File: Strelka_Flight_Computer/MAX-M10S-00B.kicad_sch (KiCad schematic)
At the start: 15 parts, among them IC2 MAX-M10S-00B

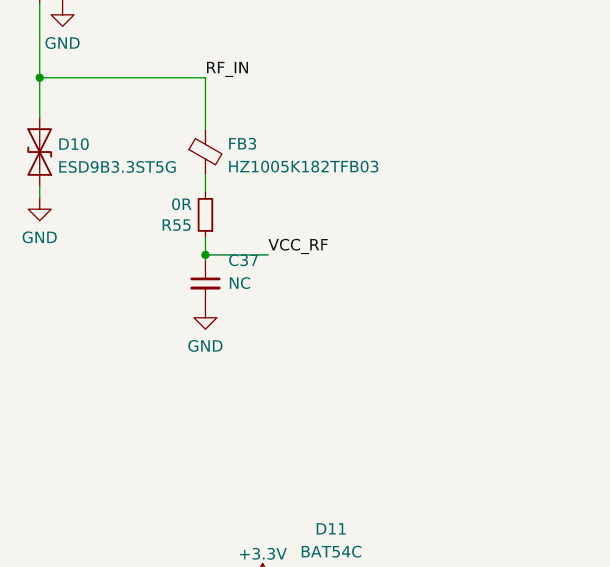
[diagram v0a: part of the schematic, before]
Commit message: Continued routing
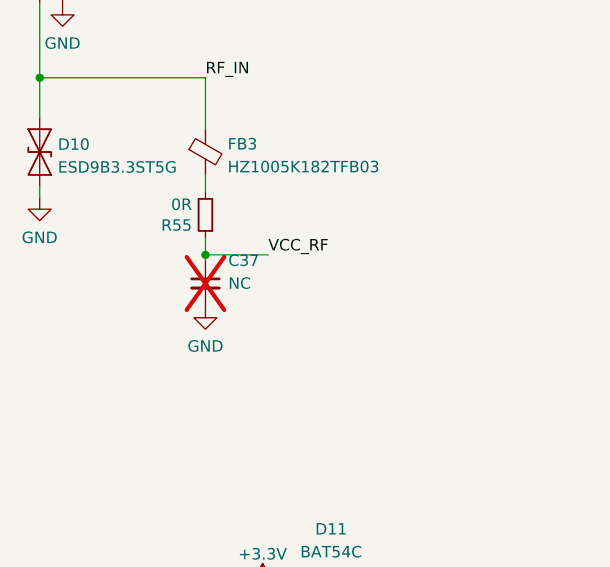
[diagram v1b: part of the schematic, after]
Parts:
- C37: now not fitted
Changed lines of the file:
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@@
   )
   (symbol (lib_id "Device:C_Small") (at 53.975 107.315 0) (unit 1)
-    (in_bom yes) (on_board yes) (dnp no)
+    (in_bom yes) (on_board yes) (dnp yes)
     (property "Reference" "C37" (at 56.515 104.775 0)
       (effects (font (size 1.27 1.27)) (justify left))

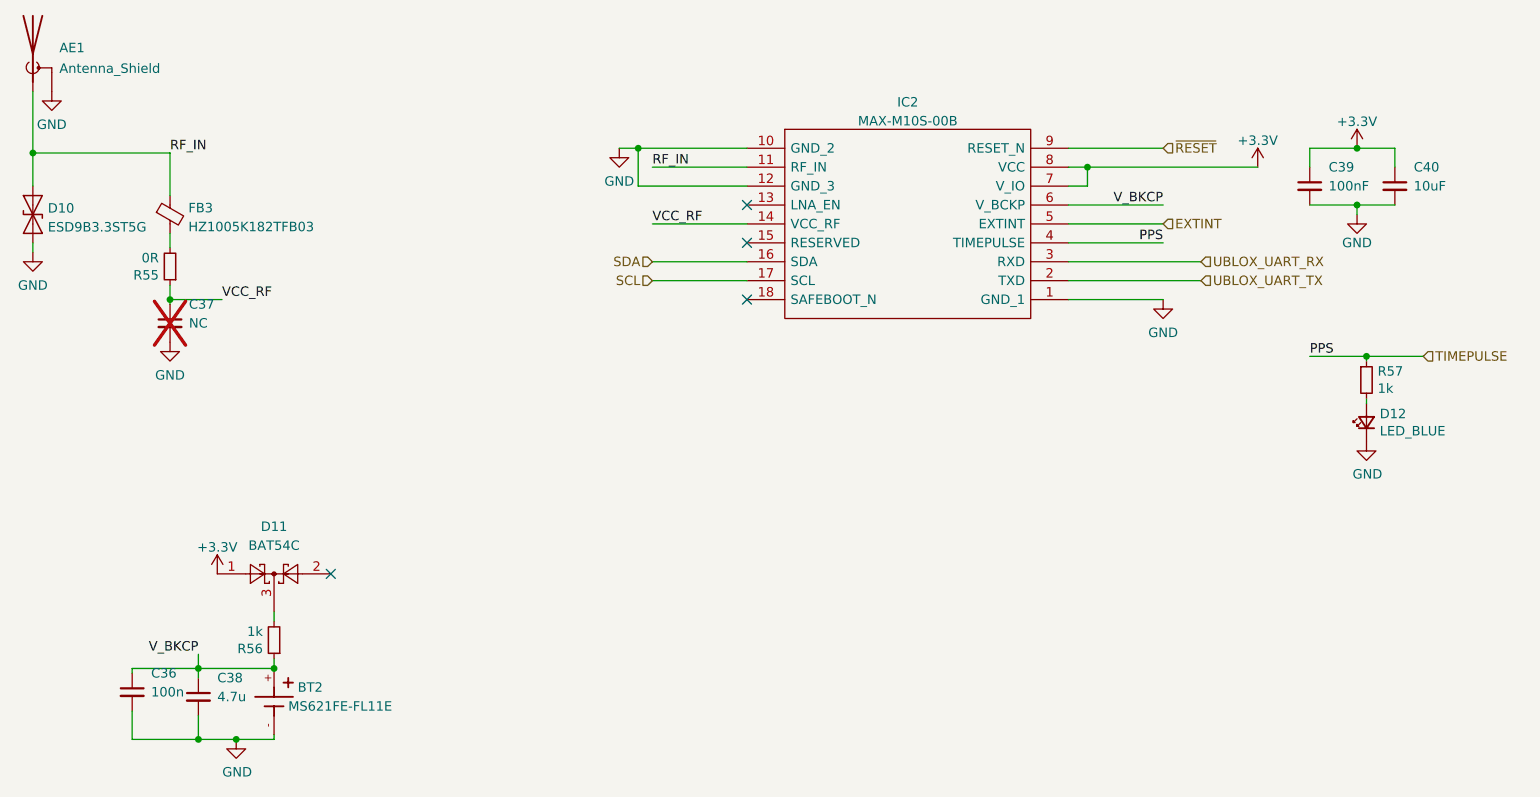
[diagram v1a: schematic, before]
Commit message: Routing complete
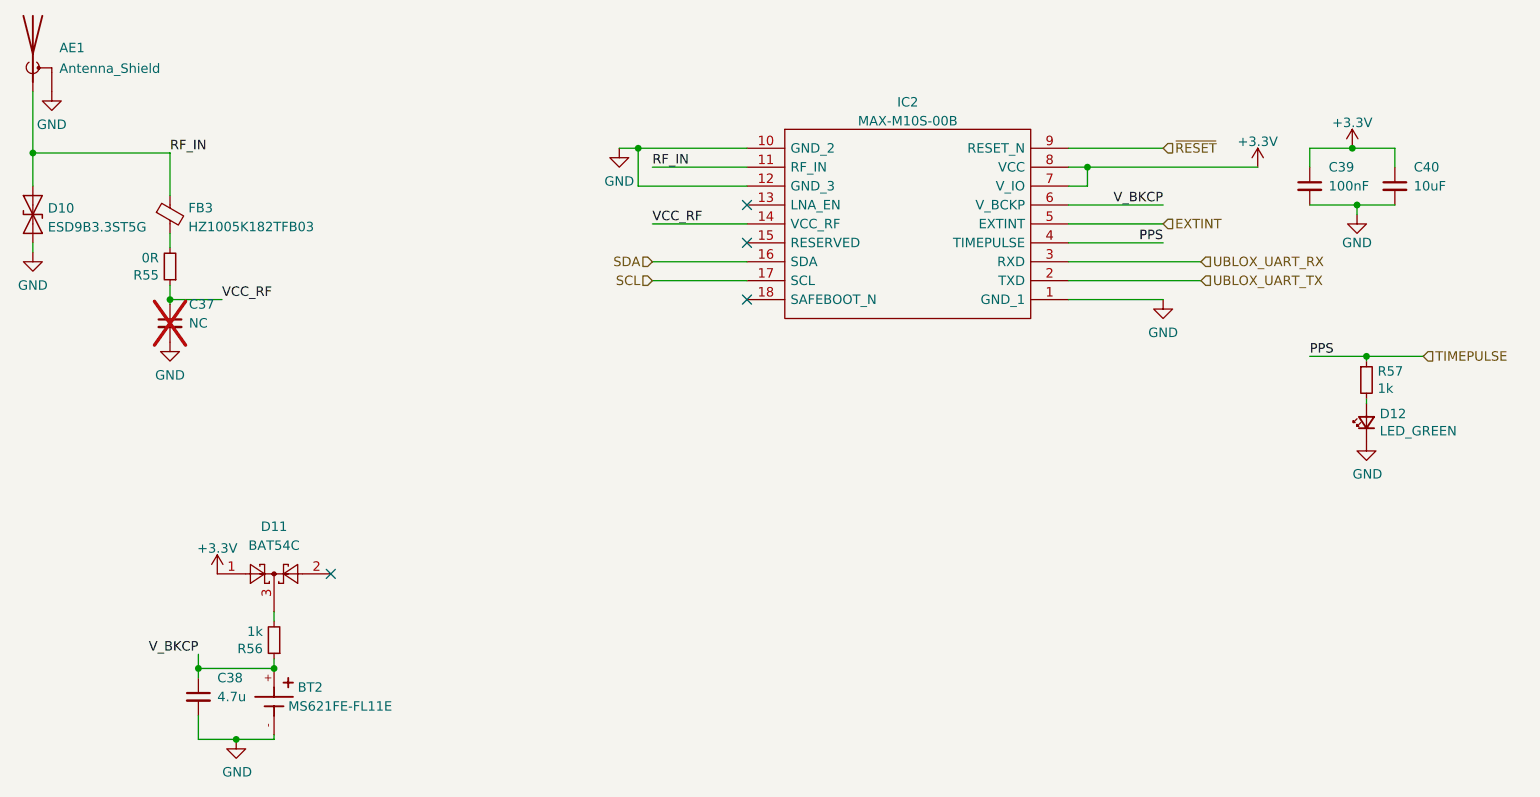
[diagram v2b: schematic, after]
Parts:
- removed C36: 100n, Capacitor_SMD:C_0402_1005Metric, symbol Device:C_Small
- D12: value LED_BLUE -> LED_GREEN; LCSC (none) -> C72043
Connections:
- net +3V3 renamed +3.3V
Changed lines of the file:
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@@
 (kicad_sch (version 20230121) (generator eeschema)
   (paper "A4")
+  (junction (at 212.725 83.82) (diameter 0) (color 0 0 0 0)
+  )
   (junction (at 177.165 86.36) (diameter 0) (color 0 0 0 0)
   )
@@
   (junction (at 213.36 91.44) (diameter 0) (color 0 0 0 0)
   )
-  (junction (at 213.36 83.82) (diameter 0) (color 0 0 0 0)
-  )
   (junction (at 57.785 153.67) (diameter 0) (color 0 0 0 0)
   )
   (junction (at 62.865 163.195) (diameter 0) (color 0 0 0 0)
-  )
-  (junction (at 57.785 163.195) (diameter 0) (color 0 0 0 0)
   )
   (junction (at 53.975 104.14) (diameter 0) (color 0 0 0 0)
@@
     (stroke (width 0) (type default))
   )
-  (wire (pts (xy 48.895 159.385) (xy 48.895 163.195))
-    (stroke (width 0) (type default))
-  )
   (wire (pts (xy 53.975 102.235) (xy 53.975 104.14))
     (stroke (width 0) (type default))
   )
-  (wire (pts (xy 48.895 163.195) (xy 57.785 163.195))
-    (stroke (width 0) (type default))
-  )
   (wire (pts (xy 53.975 104.14) (xy 60.96 104.14))
     (stroke (width 0) (type default))
@@
     (stroke (width 0) (type default))
   )
+  (wire (pts (xy 212.725 83.82) (xy 218.44 83.82))
+    (stroke (width 0) (type default))
+  )
   (wire (pts (xy 53.975 90.17) (xy 53.975 84.455))
     (stroke (width 0) (type default))
@@
     (stroke (width 0) (type default))
   )
-  (wire (pts (xy 48.895 153.67) (xy 57.785 153.67))
-    (stroke (width 0) (type default))
-  )
   (wire (pts (xy 57.785 160.02) (xy 57.785 163.195))
     (stroke (width 0) (type default))
@@
     (stroke (width 0) (type default))
   )
-  (wire (pts (xy 213.36 83.82) (xy 218.44 83.82))
+  (wire (pts (xy 207.01 83.82) (xy 212.725 83.82))
     (stroke (width 0) (type default))
   )
@@
     (stroke (width 0) (type default))
   )
-  (wire (pts (xy 48.895 154.305) (xy 48.895 153.67))
-    (stroke (width 0) (type default))
-  )
   (wire (pts (xy 57.785 153.67) (xy 67.945 153.67))
     (stroke (width 0) (type default))
@@
   )
   (wire (pts (xy 57.785 153.67) (xy 57.785 154.94))
-    (stroke (width 0) (type default))
-  )
-  (wire (pts (xy 207.01 83.82) (xy 213.36 83.82))
     (stroke (width 0) (type default))
   )
@@
         (path "/e63e39d7-6ac0-4ffd-8aa3-1841a4541b55/78f71895-bddb-4f64-a608-99074f2d1c44/139c9d95-fce8-4012-aeed-de926a08d12b"
           (reference "BT2") (unit 1)
+        )
+      )
+    )
+  )
+  (symbol (lib_name "+3.3V_1") (lib_id "power:+3.3V") (at 200.025 86.36 0) (unit 1)
+    (in_bom yes) (on_board yes) (dnp no) (fields_autoplaced)
+    (property "Reference" "#PWR015" (at 200.025 90.17 0)
+      (effects (font (size 1.27 1.27)) hide)
+    )
+    (property "Value" "+3.3V" (at 200.025 82.931 0)
+      (effects (font (size 1.27 1.27)))
+    )
+    (property "Footprint" "" (at 200.025 86.36 0)
+      (effects (font (size 1.27 1.27)) hide)
+    )
+    (property "Datasheet" "" (at 200.025 86.36 0)
+      (effects (font (size 1.27 1.27)) hide)
+    )
+    (pin "1")
+    (instances
+      (project "Strelka_Flight_Computer"
+        (path "/e63e39d7-6ac0-4ffd-8aa3-1841a4541b55/0daddb18-1491-4767-9ffd-66c8a8ce3cbd"
+          (reference "#PWR015") (unit 1)
+        )
+        (path "/e63e39d7-6ac0-4ffd-8aa3-1841a4541b55/78f71895-bddb-4f64-a608-99074f2d1c44/139c9d95-fce8-4012-aeed-de926a08d12b"
+          (reference "#PWR016") (unit 1)
         )
       )
@@
     )
   )
-  (symbol (lib_id "power:+3.3V") (at 200.025 86.36 0) (unit 1)
-    (in_bom yes) (on_board yes) (dnp no) (fields_autoplaced)
-    (property "Reference" "#PWR0210" (at 200.025 90.17 0)
-      (effects (font (size 1.27 1.27)) hide)
-    )
-    (property "Value" "+3.3V" (at 200.025 82.7842 0)
-      (effects (font (size 1.27 1.27)))
-    )
-    (property "Footprint" "" (at 200.025 86.36 0)
-      (effects (font (size 1.27 1.27)) hide)
-    )
-    (property "Datasheet" "" (at 200.025 86.36 0)
-      (effects (font (size 1.27 1.27)) hide)
-    )
-    (pin "1")
-    (instances
-      (project "Strelka_Flight_Computer"
-        (path "/e63e39d7-6ac0-4ffd-8aa3-1841a4541b55/78f71895-bddb-4f64-a608-99074f2d1c44/139c9d95-fce8-4012-aeed-de926a08d12b"
-          (reference "#PWR0210") (unit 1)
-        )
-      )
-    )
-  )
   (symbol (lib_id "Device:C_Small") (at 57.785 157.48 0) (unit 1)
     (in_bom yes) (on_board yes) (dnp no)
@@
     )
   )
-  (symbol (lib_id "power:+3.3V") (at 213.36 83.82 0) (unit 1)
-    (in_bom yes) (on_board yes) (dnp no) (fields_autoplaced)
-    (property "Reference" "#PWR0209" (at 213.36 87.63 0)
-      (effects (font (size 1.27 1.27)) hide)
-    )
-    (property "Value" "+3.3V" (at 213.36 80.2442 0)
-      (effects (font (size 1.27 1.27)))
-    )
-    (property "Footprint" "" (at 213.36 83.82 0)
-      (effects (font (size 1.27 1.27)) hide)
-    )
-    (property "Datasheet" "" (at 213.36 83.82 0)
-      (effects (font (size 1.27 1.27)) hide)
-    )
-    (pin "1")
-    (instances
-      (project "Strelka_Flight_Computer"
-        (path "/e63e39d7-6ac0-4ffd-8aa3-1841a4541b55/78f71895-bddb-4f64-a608-99074f2d1c44/139c9d95-fce8-4012-aeed-de926a08d12b"
-          (reference "#PWR0209") (unit 1)
+  (symbol (lib_name "+3.3V_1") (lib_id "power:+3.3V") (at 212.725 83.82 0) (unit 1)
+    (in_bom yes) (on_board yes) (dnp no) (fields_autoplaced)
+    (property "Reference" "#PWR015" (at 212.725 87.63 0)
+      (effects (font (size 1.27 1.27)) hide)
+    )
+    (property "Value" "+3.3V" (at 212.725 80.391 0)
+      (effects (font (size 1.27 1.27)))
+    )
+    (property "Footprint" "" (at 212.725 83.82 0)
+      (effects (font (size 1.27 1.27)) hide)
+    )
+    (property "Datasheet" "" (at 212.725 83.82 0)
+      (effects (font (size 1.27 1.27)) hide)
+    )
+    (pin "1")
+    (instances
+      (project "Strelka_Flight_Computer"
+        (path "/e63e39d7-6ac0-4ffd-8aa3-1841a4541b55/0daddb18-1491-4767-9ffd-66c8a8ce3cbd"
+          (reference "#PWR015") (unit 1)
+        )
+        (path "/e63e39d7-6ac0-4ffd-8aa3-1841a4541b55/78f71895-bddb-4f64-a608-99074f2d1c44/139c9d95-fce8-4012-aeed-de926a08d12b"
+          (reference "#PWR017") (unit 1)
         )
       )
@@
         (path "/e63e39d7-6ac0-4ffd-8aa3-1841a4541b55/78f71895-bddb-4f64-a608-99074f2d1c44/139c9d95-fce8-4012-aeed-de926a08d12b"
           (reference "#PWR0206") (unit 1)
-        )
-      )
-    )
-  )
-  (symbol (lib_id "power:+3.3V") (at 60.325 140.97 0) (unit 1)
-    (in_bom yes) (on_board yes) (dnp no) (fields_autoplaced)
-    (property "Reference" "#PWR0214" (at 60.325 144.78 0)
-      (effects (font (size 1.27 1.27)) hide)
-    )
-    (property "Value" "+3.3V" (at 60.325 137.3942 0)
-      (effects (font (size 1.27 1.27)))
-    )
-    (property "Footprint" "" (at 60.325 140.97 0)
-      (effects (font (size 1.27 1.27)) hide)
-    )
-    (property "Datasheet" "" (at 60.325 140.97 0)
-      (effects (font (size 1.27 1.27)) hide)
-    )
-    (pin "1")
-    (instances
-      (project "Strelka_Flight_Computer"
-        (path "/e63e39d7-6ac0-4ffd-8aa3-1841a4541b55/78f71895-bddb-4f64-a608-99074f2d1c44/139c9d95-fce8-4012-aeed-de926a08d12b"
-          (reference "#PWR0214") (unit 1)
         )
       )
@@
     )
   )
-  (symbol (lib_id "Device:C_Small") (at 48.895 156.845 0) (unit 1)
-    (in_bom yes) (on_board yes) (dnp no)
-    (property "Reference" "C36" (at 51.435 154.305 0)
-      (effects (font (size 1.27 1.27)) (justify left))
-    )
-    (property "Value" "100n" (at 51.435 156.845 0)
-      (effects (font (size 1.27 1.27)) (justify left))
-    )
-    (property "Footprint" "Capacitor_SMD:C_0402_1005Metric" (at 48.895 156.845 0)
-      (effects (font (size 1.27 1.27)) hide)
-    )
-    (property "Datasheet" "~" (at 48.895 156.845 0)
-      (effects (font (size 1.27 1.27)) hide)
-    )
-    (pin "1")
-    (pin "2")
-    (instances
-      (project "Strelka_Flight_Computer"
-        (path "/e63e39d7-6ac0-4ffd-8aa3-1841a4541b55/78f71895-bddb-4f64-a608-99074f2d1c44/139c9d95-fce8-4012-aeed-de926a08d12b"
-          (reference "C36") (unit 1)
-        )
-      )
-    )
-  )
   (symbol (lib_id "Device:LED_Small") (at 214.63 120.65 90) (unit 1)
     (in_bom yes) (on_board yes) (dnp no)
@@
       (effects (font (size 1.27 1.27)) (justify right))
     )
-    (property "Value" "LED_BLUE" (at 216.408 121.793 90)
+    (property "Value" "LED_GREEN" (at 216.408 121.793 90)
       (effects (font (size 1.27 1.27)) (justify right))
     )
@@
       (effects (font (size 1.27 1.27)) hide)
     )
+    (property "LCSC" "C72043" (at 214.63 120.65 90)
+      (effects (font (size 1.27 1.27)) hide)
+    )
     (pin "1")
     (pin "2")
@@
         )
       )
+    )
+  )
+  (symbol (lib_name "+3.3V_1") (lib_id "power:+3.3V") (at 60.325 140.97 0) (unit 1)
+    (in_bom yes) (on_board yes) (dnp no) (fields_autoplaced)
+    (property "Reference" "#PWR015" (at 60.325 144.78 0)
+      (effects (font (size 1.27 1.27)) hide)
+    )
+    (property "Value" "+3.3V" (at 60.325 137.541 0)
+      (effects (font (size 1.27 1.27)))
+    )
+    (property "Footprint" "" (at 60.325 140.97 0)
+      (effects (font (size 1.27 1.27)) hide)
+    )
+    (property "Datasheet" "" (at 60.325 140.97 0)
+      (effects (font (size 1.27 1.27)) hide)
+    )
+    (pin "1")
+    (instances
+      (project "Strelka_Flight_Computer"
+        (path "/e63e39d7-6ac0-4ffd-8aa3-1841a4541b55/0daddb18-1491-4767-9ffd-66c8a8ce3cbd"
+          (reference "#PWR015") (unit 1)
+        )
+        (path "/e63e39d7-6ac0-4ffd-8aa3-1841a4541b55/78f71895-bddb-4f64-a608-99074f2d1c44/139c9d95-fce8-4012-aeed-de926a08d12b"
+          (reference "#PWR018") (unit 1)
+        )
+      )
